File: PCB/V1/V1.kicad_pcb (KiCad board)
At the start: 2 copper layers, 40 x 46.2 mm, 35 parts, among them IC1 TMP112NAIDRLR, J1 Conn_02x06_Odd_Even, J2 Conn_02x06_Odd_Even, J3 USB_B_Micro, J4 Programmer, SW1 SW_Push, U1 MPU6050, U2 MDBT50Q-1MV2, U3 MAX6372, Y1 32.768kHz

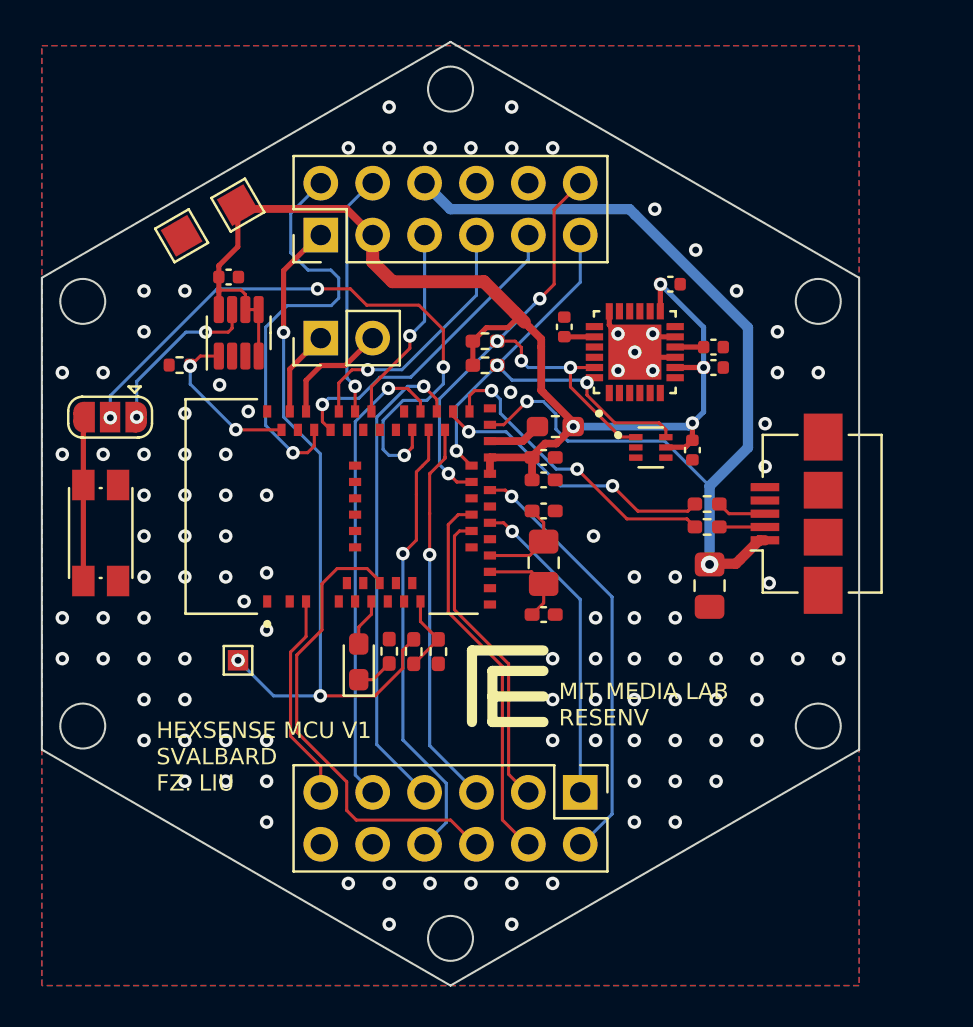
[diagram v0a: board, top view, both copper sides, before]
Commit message: udated by FZ
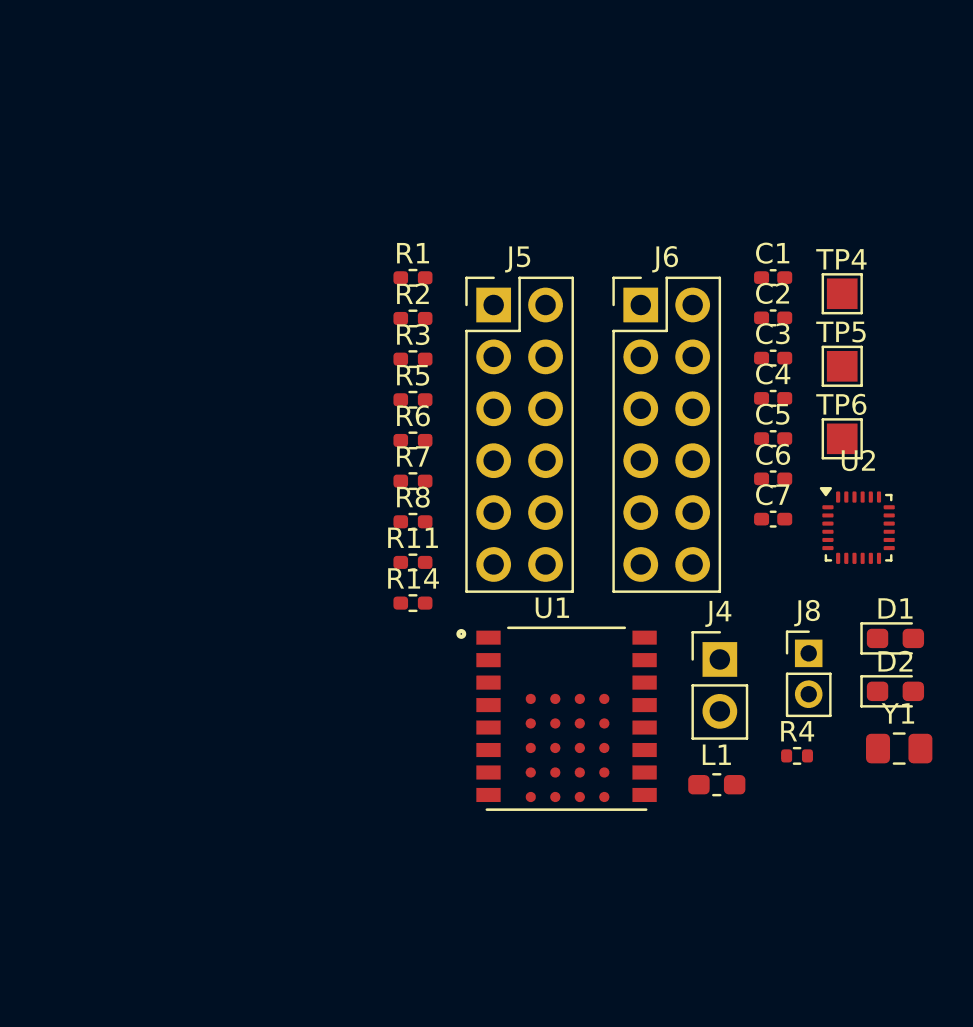
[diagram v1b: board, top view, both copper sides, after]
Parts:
- removed C10, C11: 0.1uF, Capacitor_SMD:C_0402_1005Metric
- removed C8: 2200pF, Capacitor_SMD:C_0402_1005Metric
- removed C9: 47uF, Capacitor_SMD:C_0805_2012Metric_Pad1.18x1.45mm_HandSolder
- removed IC1: TMP112NAIDRLR, Mylib:SOT50P160X60-6N
- removed J1, J2: Conn_02x06_Odd_Even, Connector_PinHeader_2.54mm:PinHeader_2x06_P2.54mm_Vertical
- removed J3: USB_B_Micro, Connector_USB:USB_Micro-B_Amphenol_10104110_Horizontal
- removed JP1: RST Jumper, Jumper:SolderJumper-3_P1.3mm_Open_RoundedPad1.0x1.5mm
- removed SW1: SW_Push, Button_Switch_SMD:SW_Push_1P1T_NO_CK_KMR2
- removed TP1: VCC_TP, TestPoint:TestPoint_Pad_1.5x1.5mm
- removed TP2: GND_TP, TestPoint:TestPoint_Pad_1.5x1.5mm
- removed TP3: BAT_TP, TestPoint:TestPoint_Pad_1.0x1.0mm
- removed U3: MAX6372, Package_TO_SOT_SMD:SOT-23-8
- added D2: LED, Diode_SMD:D_0603_1608Metric_Pad1.05x0.95mm_HandSolder, F.Cu at (171.9, 108.8)
- added J5: Conn_02x06_Odd_Even, Connector_PinHeader_2.54mm:PinHeader_2x06_P2.54mm_Vertical, F.Cu at (152.3, 89.9)
- added J6: Conn_02x06_Odd_Even, Connector_PinHeader_2.54mm:PinHeader_2x06_P2.54mm_Vertical, F.Cu at (159.5, 89.9)
- added J8: RESET, Connector_PinHeader_2.00mm:PinHeader_1x02_P2.00mm_Vertical, F.Cu at (167.7, 106.9)
- added R14: 330, Resistor_SMD:R_0402_1005Metric_Pad0.72x0.64mm_HandSolder, F.Cu at (148.3, 104.5)
- added R3: 10K, Resistor_SMD:R_0402_1005Metric_Pad0.72x0.64mm_HandSolder, F.Cu at (148.3, 92.5)
- added TP4: TestPoint, TestPoint:TestPoint_Pad_1.5x1.5mm, F.Cu at (169.3, 89.3)
- added TP5: TestPoint, TestPoint:TestPoint_Pad_1.5x1.5mm, F.Cu at (169.3, 92.9)
- added TP6: TestPoint, TestPoint:TestPoint_Pad_1.5x1.5mm, F.Cu at (169.3, 96.4)
- C1, C7: footprint Capacitor_SMD:C_0402_1005Metric -> Capacitor_SMD:C_0402_1005Metric_Pad0.74x0.62mm_HandSolder
- C3: value 10000pF -> 0.1uF; footprint Capacitor_SMD:C_0402_1005Metric -> Capacitor_SMD:C_0402_1005Metric_Pad0.74x0.62mm_HandSolder
- R5, R6: value 27 -> 10K
- U1: value MPU6050 -> BC832; footprint Mylib:IC_MPU6050 -> Mylib:XCVR_BC832
- U2: value MDBT50Q-1MV2 -> ICM-20948; footprint Mylib:XCVR_MDBT50Q-1MV2 -> Sensor_Motion:InvenSense_QFN-24_3x3mm_P0.4mm
- moved R4 35.8 mm to (167.1, 112.0), turned to 0 degrees
- moved D1 26.3 mm to (171.9, 106.2), turned to 0 degrees
- moved U2 25.2 mm to (170.1, 100.8), turned to 0 degrees
- moved J4 25.1 mm to (163.3, 107.2), turned to 0 degrees
- moved Y1 19.6 mm to (172.1, 111.6), turned to 0 degrees
- moved L1 19.2 mm to (163.2, 113.4), turned to 0 degrees
- moved C2 18.4 mm to (166.0, 90.5), turned to 0 degrees
- moved U1 18.2 mm to (155.8, 110.1), turned to 0 degrees
- moved R5 15.3 mm to (148.3, 94.5)
- moved R6 15.0 mm to (148.3, 96.5)
- moved C4 12.5 mm to (166.0, 94.5), turned to 0 degrees
- moved C5 11.3 mm to (166.0, 96.4), turned to 0 degrees
- moved C6 11.2 mm to (166.0, 98.4), turned to 0 degrees
- moved C7 8.91 mm to (166.0, 100.4), turned to 0 degrees
- moved R7 8.34 mm to (148.3, 98.5), turned to 0 degrees
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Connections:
- C1 pad 1: GND -> Net-(U2-REGOUT)
- C1 pad 2: VCC -> GND
- C2 pad 2: Net-(U2-P0.00/XL1) -> Net-(U1-P00/XL1)
- C3 pad 1: GND -> +1V8
- C3 pad 2: VCC -> GND
- C4 pad 2: Net-(U2-P0.01/XL2) -> Net-(U1-P01/XL2)
- C7 pad 1: GND -> /D10
- C7 pad 2: Net-(U1-REGOUT) -> GND
- L1 pad 2: Net-(U2-DCCH) -> unconnected-(L1-Pad2)
- R5 pad 1: /USB+ -> /SCL_1V8
- R5 pad 2: Net-(J3-D+) -> +1V8
- R6 pad 1: /USB- -> /SDA_1V8
- R6 pad 2: Net-(J3-D-) -> +1V8
- U1 pad 10: Net-(U1-REGOUT) -> unconnected-(U1-P21/RESET-Pad10)
- U1 pad 11: GND -> Net-(U1-P00/XL1)
- U1 pad 12: unconnected-(U1-INT-Pad12) -> Net-(U1-P01/XL2)
- U1 pad 13: VCC -> unconnected-(U1-P02/AIN0-Pad13)
- U1 pad 3: unconnected-(U1-NC3-Pad3) -> /SWDIO
- U1 pad 4: unconnected-(U1-NC4-Pad4) -> /SWDCLK
- U1 pad 8: VCC -> unconnected-(U1-P12/TX-Pad8)
- U1 pad 9: GND -> unconnected-(U1-P03/AIN1-Pad9)
- U2 pad 1: GND -> unconnected-(U2-NC-Pad1)
- U2 pad 10: unconnected-(U2-P0.29/AIN5-Pad10) -> Net-(U2-REGOUT)
- U2 pad 11: /A4 -> GND
- U2 pad 13: /A3 -> +1V8
- U2 pad 14: /A2 -> unconnected-(U2-NC-Pad14)
- U2 pad 15: GND -> unconnected-(U2-NC-Pad15)
- U2 pad 16: /D10 -> unconnected-(U2-NC-Pad16)
- U2 pad 17: Net-(U2-P0.00/XL1) -> unconnected-(U2-NC-Pad17)
- U2 pad 18: Net-(U2-P0.01/XL2) -> GND
- U2 pad 19: /D9 -> unconnected-(U2-RESV_19-Pad19)
- U2 pad 2: GND -> unconnected-(U2-NC-Pad2)
- U2 pad 20: /A0 -> GND
- U2 pad 21: /A1 -> unconnected-(U2-AUX_DA-Pad21)
- U2 pad 22: /D11 -> Net-(U2-~{CS})
- U2 pad 23: /D6 -> /SCL_1V8
- U2 pad 24: /D12 -> /SDA_1V8
- U2 pad 3: /LED2 -> unconnected-(U2-NC-Pad3)
- U2 pad 8: /LED1 -> +1V8
- U2 pad 9: /A5 -> GND
- Y1 pad 1: Net-(U2-P0.01/XL2) -> Net-(U1-P01/XL2)
- Y1 pad 2: Net-(U2-P0.00/XL1) -> Net-(U1-P00/XL1)
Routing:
- net VCC: track 63.3 -> 0.00 mm, vias 4 -> 0
- net +5V: track 47.7 -> 0.00 mm, vias 2 -> 0
- net /VBAT: track 35.1 -> 0.00 mm, vias 3 -> 0
- net /~{RESET}: track 30.7 -> 0.00 mm, vias 4 -> 0
- net /SCL: track 29.4 -> 0.00 mm, vias 5 -> 0
- net /SDA: track 24.5 -> 0.00 mm, vias 3 -> 0
- net /MOSI: track 23.8 -> 0.00 mm, vias 1 -> 0
- net /A5: track 23.2 -> 0.00 mm
- net /MISO: track 23.1 -> 0.00 mm, vias 1 -> 0
- net /~{CS}: track 22.1 -> 0.00 mm, vias 1 -> 0
- net /D13: track 21.0 -> 0.00 mm, vias 1 -> 0
- net /~{EN}: track 20.7 -> 0.00 mm, vias 1 -> 0
- net /SCK: track 19.0 -> 0.00 mm, vias 1 -> 0
- net /D6: track 18.7 -> 0.00 mm
- net /TXD: track 15.6 -> 0.00 mm, vias 1 -> 0
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- removed copper zone on B.Cu, net GND
- removed copper zone on F.Cu, net GND
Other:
- board outline removed
- board text removed: "HEXSENSE MCU V1 SVALBARD FZ. LIU"
- board text removed: "MIT MEDIA LAB RESENV"
